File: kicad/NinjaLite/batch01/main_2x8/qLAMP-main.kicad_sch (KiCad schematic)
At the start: 17 parts, among them Q3 Q_NMOS_GSD, Q5 Q_NMOS_GSD, U17 LITE_LCD, U5 ESP32-WROOM-32, U6 ESP32-WROOM-32U

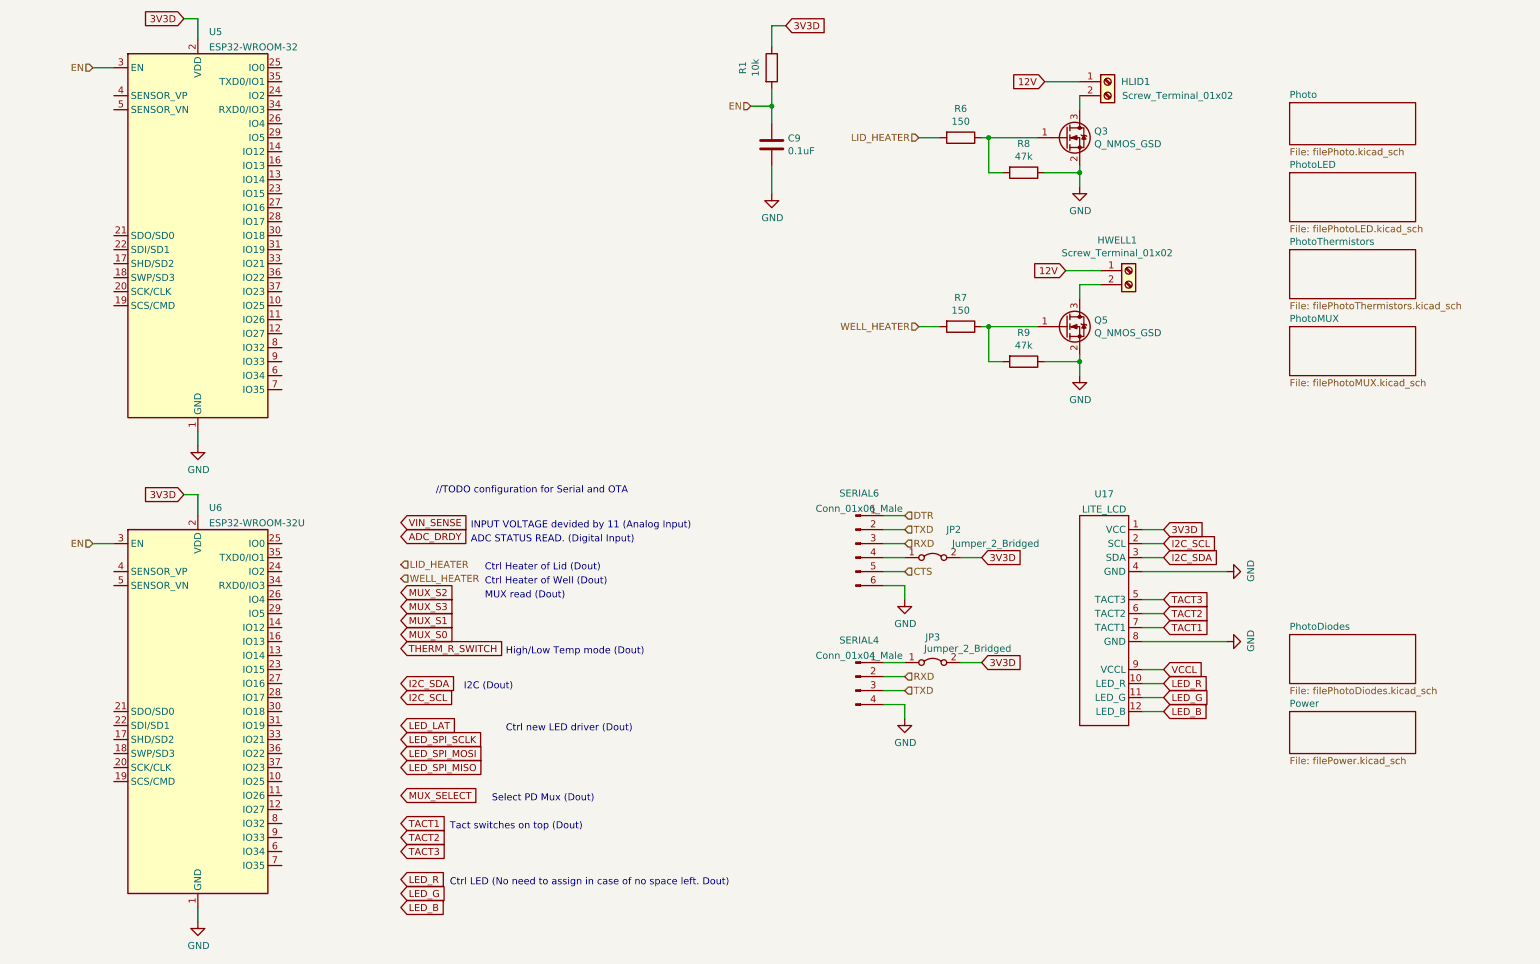
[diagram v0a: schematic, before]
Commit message: wiring
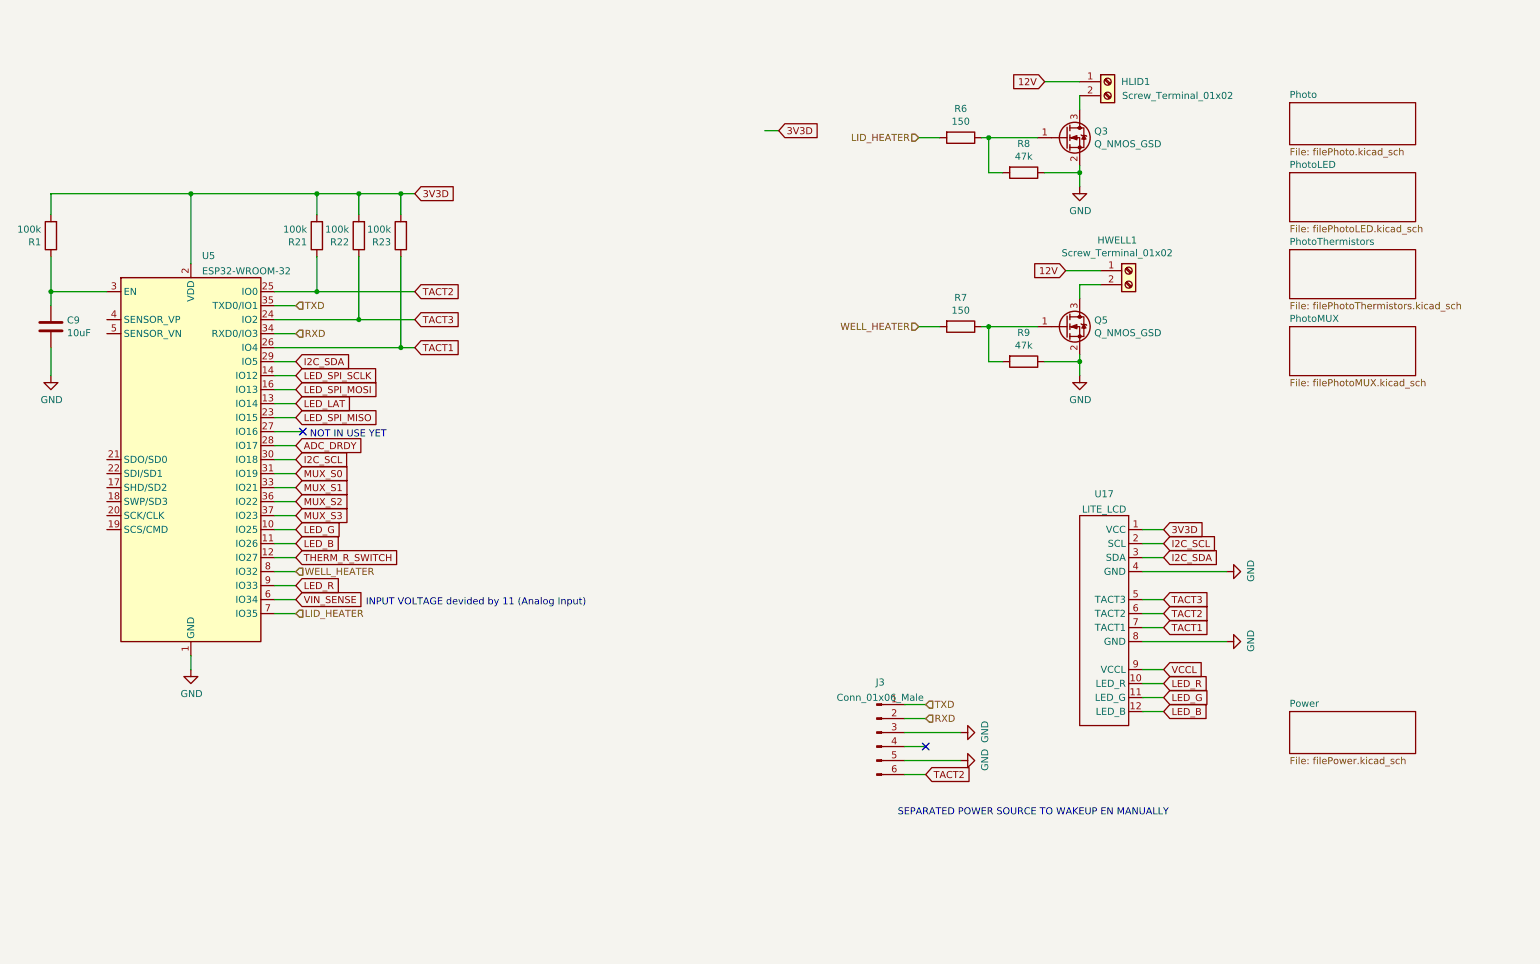
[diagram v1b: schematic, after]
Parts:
- removed JP2, JP3: Jumper_2_Bridged, Jumper:SolderJumper-2_P1.3mm_Open_TrianglePad1.0x1.5mm, symbol Jumper:Jumper_2_Bridged
- removed SERIAL4: Conn_01x04_Male, Connector_PinSocket_2.54mm:PinSocket_1x04_P2.54mm_Vertical, symbol Connector:Conn_01x04_Male
- removed SERIAL6: Conn_01x06_Male, Connector_PinSocket_2.54mm:PinSocket_1x06_P2.54mm_Vertical, symbol Connector:Conn_01x06_Male
- removed U6: ESP32-WROOM-32U, RF_Module:ESP32-WROOM-32U, symbol RF_Module:ESP32-WROOM-32U
- added J3: Conn_01x06_Male, Connector_PinHeader_2.54mm:PinHeader_1x06_P2.54mm_Vertical, symbol Connector:Conn_01x06_Male
- added R21, R22, R23: 100k, Resistor_SMD:R_0603_1608Metric, symbol Device:R
- C9: value 0.1uF -> 10uF; footprint Capacitor_SMD:C_0603_1608Metric -> Capacitor_SMD:C_0805_2012Metric
- R1: value 10k -> 100k
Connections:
- net 3V3D: now also R1.2, R21.2, R22.2, R23.2; no longer R1.1
- net ADC_DRDY: now also U5.28 (IO17)
- net GND: now also J3.3 (Pin_3), J3.5 (Pin_5)
- net I2C_SCL: now also U5.30 (IO18)
- net I2C_SDA: now also U5.29 (IO5)
- net LED_B: now also U5.11 (IO26)
- net LED_G: now also U5.10 (IO25)
- net LED_LAT: now also U5.13 (IO14)
- net LED_R: now also U5.9 (IO33)
- net LED_SPI_MISO: now also U5.23 (IO15)
- net LED_SPI_MOSI: now also U5.16 (IO13)
- net LED_SPI_SCLK: now also U5.14 (IO12)
- net LID_HEATER: now also U5.7 (IO35)
- net MUX_S0: now also U5.31 (IO19)
- net MUX_S1: now also U5.33 (IO21)
- net MUX_S2: now also U5.36 (IO22)
- net MUX_S3: now also U5.37 (IO23)
- net RXD: now also U5.34 (RXD0/IO3), J3.2 (Pin_2)
- net TACT1: now also U5.26 (IO4), R23.1
- net TACT2: now also U5.25 (IO0), J3.6 (Pin_6), R21.1
- net TACT3: now also U5.24 (IO2), R22.1
- net THERM_R_SWITCH: now also U5.12 (IO27)
- net TXD: now also U5.35 (TXD0/IO1), J3.1 (Pin_1)
- net VIN_SENSE: now also U5.6 (IO34)
- net WELL_HEATER: now also U5.8 (IO32)
- net EN: no longer names the net of C9.1, U5.3 (EN)
- net EN: now also R1.1; no longer R1.2
- no-connect marks 0 -> 2
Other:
- removed sheet PhotoDiodes
- note added: "NOT IN USE YET"
- note added: "SEPARATED POWER SOURCE TO WAKEUP EN MANUALLY"
- note removed: "//TODO configuration for Serial and OTA"
- note removed: "ADC STATUS READ. (Digital Input)"
- note removed: "Ctrl Heater of Lid (Dout)"
- note removed: "Ctrl Heater of Well (Dout)"
- note removed: "Ctrl LED (No need to assign in case of no space left. Dout)"
- note removed: "Ctrl new LED driver (Dout)"
- note removed: "High/Low Temp mode (Dout)"
- note removed: "I2C (Dout)"
- note removed: "MUX read (Dout)"
- note removed: "Select PD Mux (Dout)"
- note removed: "Tact switches on top (Dout)"
- moved on the sheet: U5

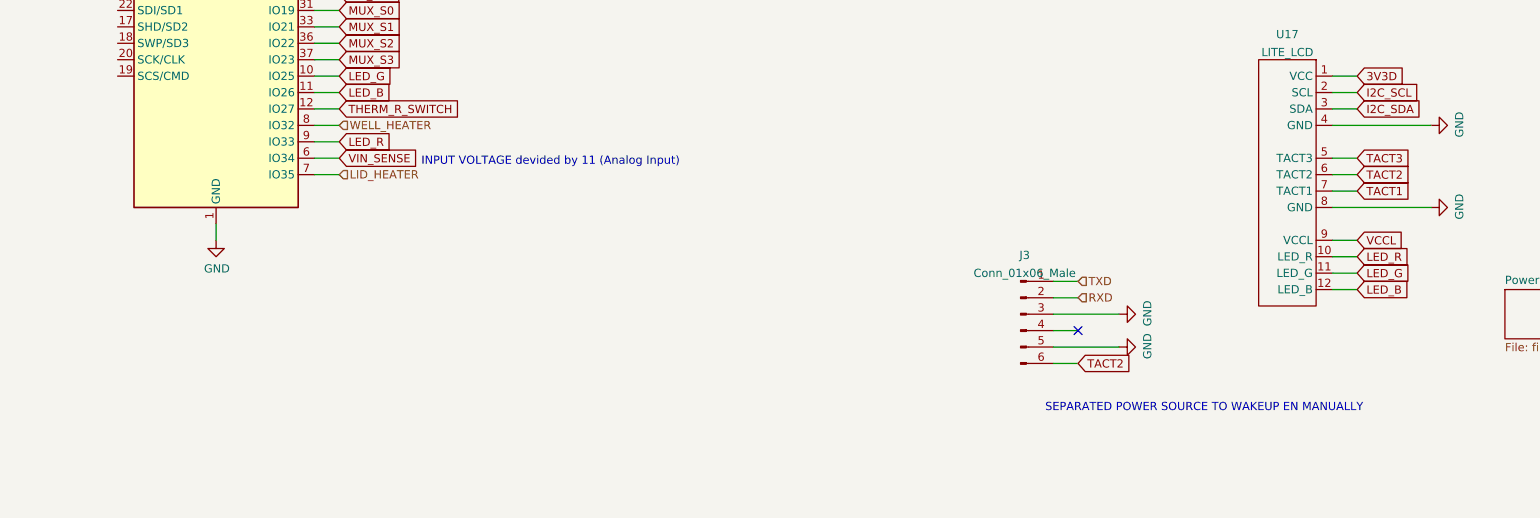
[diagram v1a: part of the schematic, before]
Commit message: sync
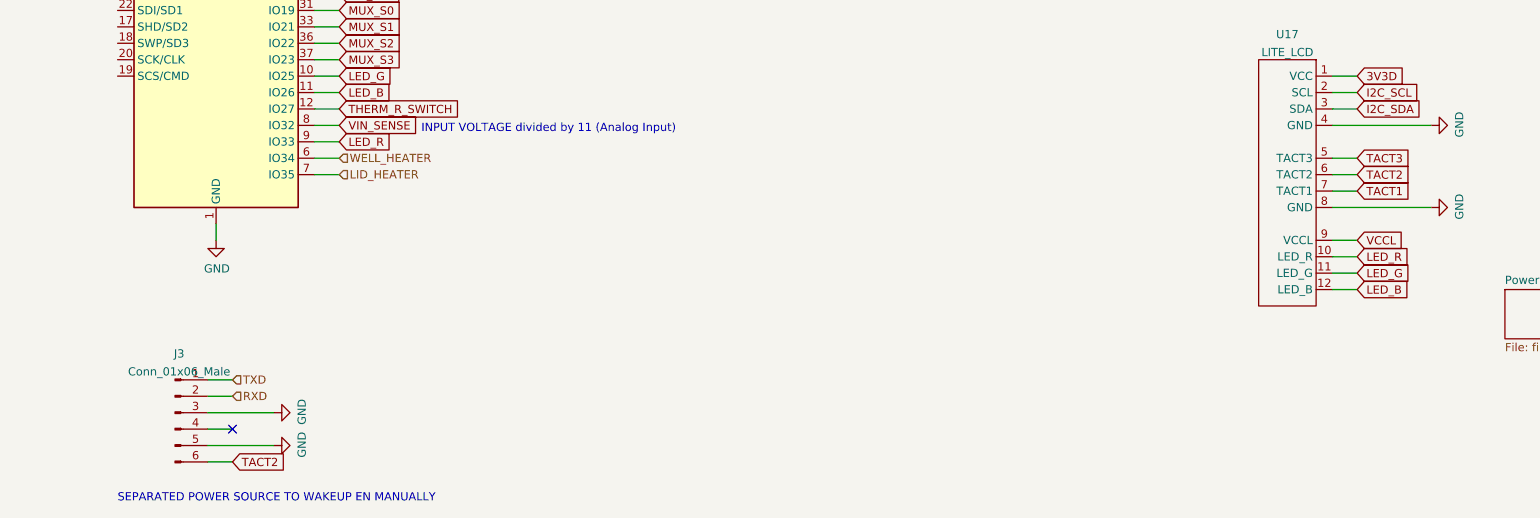
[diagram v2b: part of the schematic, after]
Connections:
- net VIN_SENSE: now also U5.8 (IO32); no longer U5.6 (IO34)
- net WELL_HEATER: now also U5.6 (IO34); no longer U5.8 (IO32)
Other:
- note added: "INPUT VOLTAGE divided by 11 (Analog Input)"
- note removed: "INPUT VOLTAGE devided by 11 (Analog Input)"
- moved on the sheet: J3
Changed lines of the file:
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@@
   (junction (at 71.12 69.85) (diameter 0) (color 0 0 0 0)
   )
-  (no_connect (at 181.61 152.4))
+  (no_connect (at 50.8 167.64))
   (no_connect (at 68.58 95.25))
-  (wire (pts (xy 177.8 149.86) (xy 187.96 149.86))
+  (wire (pts (xy 46.99 165.1) (xy 57.15 165.1))
     (stroke (width 0) (type default) (color 0 0 0 0))
   )
@@
     (stroke (width 0) (type default) (color 0 0 0 0))
   )
-  (wire (pts (xy 177.8 157.48) (xy 181.61 157.48))
+  (wire (pts (xy 46.99 172.72) (xy 50.8 172.72))
     (stroke (width 0) (type default) (color 0 0 0 0))
   )
@@
     (stroke (width 0) (type default) (color 0 0 0 0))
   )
-  (wire (pts (xy 177.8 154.94) (xy 187.96 154.94))
+  (wire (pts (xy 46.99 170.18) (xy 57.15 170.18))
     (stroke (width 0) (type default) (color 0 0 0 0))
   )
@@
     (stroke (width 0) (type default) (color 0 0 0 0))
   )
-  (wire (pts (xy 177.8 152.4) (xy 181.61 152.4))
+  (wire (pts (xy 46.99 167.64) (xy 50.8 167.64))
     (stroke (width 0) (type default) (color 0 0 0 0))
   )
@@
     (stroke (width 0) (type default) (color 0 0 0 0))
   )
-  (wire (pts (xy 177.8 147.32) (xy 181.61 147.32))
+  (wire (pts (xy 46.99 162.56) (xy 50.8 162.56))
     (stroke (width 0) (type default) (color 0 0 0 0))
   )
@@
     (stroke (width 0) (type default) (color 0 0 0 0))
   )
-  (wire (pts (xy 177.8 144.78) (xy 181.61 144.78))
+  (wire (pts (xy 46.99 160.02) (xy 50.8 160.02))
     (stroke (width 0) (type default) (color 0 0 0 0))
   )
@@
     (stroke (width 0) (type default) (color 0 0 0 0))
   )
-  (text "SEPARATED POWER SOURCE TO WAKEUP EN MANUALLY" (at 176.53 165.1 0)
+  (text "SEPARATED POWER SOURCE TO WAKEUP EN MANUALLY" (at 33.02 179.07 0)
     (effects (font (size 1.27 1.27)) (justify left bottom))
   )
@@
     (effects (font (size 1.27 1.27)) (justify left bottom))
   )
-  (text "INPUT VOLTAGE devided by 11 (Analog Input)" (at 80.01 127 0)
+  (text "INPUT VOLTAGE divided by 11 (Analog Input)" (at 80.01 121.92 0)
     (effects (font (size 1.27 1.27)) (justify left bottom))
   )
@@
     )
   )
-  (global_label "TACT2" (shape input) (at 181.61 157.48 0) (fields_autoplaced)
-    (effects (font (size 1.27 1.27)) (justify left))
-    (property "Intersheet References" "${INTERSHEET_REFS}" (id 0) (at 189.4375 157.4006 0)
+  (global_label "TACT2" (shape input) (at 50.8 172.72 0) (fields_autoplaced)
+    (effects (font (size 1.27 1.27)) (justify left))
+    (property "Intersheet References" "${INTERSHEET_REFS}" (id 0) (at 58.6275 172.6406 0)
       (effects (font (size 1.27 1.27)) (justify left) hide)
     )
@@
     )
   )
-  (global_label "VIN_SENSE" (shape input) (at 67.31 125.73 0) (fields_autoplaced)
-    (effects (font (size 1.27 1.27)) (justify left))
-    (property "Intersheet References" "${INTERSHEET_REFS}" (id 0) (at 106.68 175.26 0)
+  (global_label "VIN_SENSE" (shape input) (at 67.31 120.65 0) (fields_autoplaced)
+    (effects (font (size 1.27 1.27)) (justify left))
+    (property "Intersheet References" "${INTERSHEET_REFS}" (id 0) (at 106.68 170.18 0)
       (effects (font (size 1.27 1.27)) hide)
     )
@@
     )
   )
-  (hierarchical_label "WELL_HEATER" (shape input) (at 67.31 120.65 0)
-    (effects (font (size 1.27 1.27)) (justify left))
-  )
-  (hierarchical_label "RXD" (shape input) (at 181.61 147.32 0)
+  (hierarchical_label "WELL_HEATER" (shape input) (at 67.31 125.73 0)
+    (effects (font (size 1.27 1.27)) (justify left))
+  )
+  (hierarchical_label "RXD" (shape input) (at 50.8 162.56 0)
     (effects (font (size 1.27 1.27)) (justify left))
   )
@@
     (effects (font (size 1.27 1.27)) (justify right))
   )
-  (hierarchical_label "TXD" (shape input) (at 181.61 144.78 0)
+  (hierarchical_label "TXD" (shape input) (at 50.8 160.02 0)
     (effects (font (size 1.27 1.27)) (justify left))
   )
@@
     (pin "1")
   )
-  (symbol (lib_id "power:GND") (at 187.96 154.94 90) (unit 1)
-    (in_bom yes) (on_board yes)
-    (property "Reference" "#PWR0101" (id 0) (at 194.31 154.94 0)
-      (effects (font (size 1.27 1.27)) hide)
-    )
-    (property "Value" "GND" (id 1) (at 192.3542 154.813 0))
-    (property "Footprint" "" (id 2) (at 187.96 154.94 0)
-      (effects (font (size 1.27 1.27)) hide)
-    )
-    (property "Datasheet" "" (id 3) (at 187.96 154.94 0)
+  (symbol (lib_id "power:GND") (at 57.15 170.18 90) (unit 1)
+    (in_bom yes) (on_board yes)
+    (property "Reference" "#PWR0101" (id 0) (at 63.5 170.18 0)
+      (effects (font (size 1.27 1.27)) hide)
+    )
+    (property "Value" "GND" (id 1) (at 61.5442 170.053 0))
+    (property "Footprint" "" (id 2) (at 57.15 170.18 0)
+      (effects (font (size 1.27 1.27)) hide)
+    )
+    (property "Datasheet" "" (id 3) (at 57.15 170.18 0)
       (effects (font (size 1.27 1.27)) hide)
     )
@@
     (pin "2")
   )
-  (symbol (lib_id "Connector:Conn_01x06_Male") (at 172.72 149.86 0) (unit 1)
+  (symbol (lib_id "Connector:Conn_01x06_Male") (at 41.91 165.1 0) (unit 1)
     (in_bom yes) (on_board yes) (fields_autoplaced)
-    (property "Reference" "J3" (id 0) (at 173.355 140.7373 0))
-    (property "Value" "Conn_01x06_Male" (id 1) (at 173.355 143.5124 0))
-    (property "Footprint" "Connector_PinHeader_2.54mm:PinHeader_1x06_P2.54mm_Vertical" (id 2) (at 172.72 149.86 0)
-      (effects (font (size 1.27 1.27)) hide)
-    )
-    (property "Datasheet" "~" (id 3) (at 172.72 149.86 0)
+    (property "Reference" "J3" (id 0) (at 42.545 155.9773 0))
+    (property "Value" "Conn_01x06_Male" (id 1) (at 42.545 158.7524 0))
+    (property "Footprint" "Connector_PinHeader_2.54mm:PinHeader_1x06_P2.54mm_Vertical" (id 2) (at 41.91 165.1 0)
+      (effects (font (size 1.27 1.27)) hide)
+    )
+    (property "Datasheet" "~" (id 3) (at 41.91 165.1 0)
       (effects (font (size 1.27 1.27)) hide)
     )
@@
     (pin "9")
   )
-  (symbol (lib_id "power:GND") (at 187.96 149.86 90) (unit 1)
-    (in_bom yes) (on_board yes)
-    (property "Reference" "#PWR0102" (id 0) (at 194.31 149.86 0)
-      (effects (font (size 1.27 1.27)) hide)
-    )
-    (property "Value" "GND" (id 1) (at 192.3542 149.733 0))
-    (property "Footprint" "" (id 2) (at 187.96 149.86 0)
-      (effects (font (size 1.27 1.27)) hide)
-    )
-    (property "Datasheet" "" (id 3) (at 187.96 149.86 0)
-      (effects (font (size 1.27 1.27)) hide)
-    )
+  (symbol (lib_id "power:GND") (at 57.15 165.1 90) (unit 1)
+    (in_bom yes) (on_board yes)
+    (property "Reference" "#PWR0102" (id 0) (at 63.5 165.1 0)
+      (effects (font (size 1.27 1.27)) hide)
+    )
+    (property "Value" "GND" (id 1) (at 61.5442 164.973 0))
+    (property "Footprint" "" (id 2) (at 57.15 165.1 0)
+      (effects (font (size 1.27 1.27)) hide)
+    )
+    (property "Datasheet" "" (id 3) (at 57.15 165.1 0)
+      (effects (font (size 1.27 1.27)) hide)
+    )
